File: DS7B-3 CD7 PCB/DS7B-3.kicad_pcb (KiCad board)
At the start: 2 copper layers, 154 x 46.5 mm, 19 parts, among them CON1 Power Connector, CON4 PANASONIC, CON5 SONY, J1 COM. PORT, U2 4040, U3 74LS04, U4 74LS244

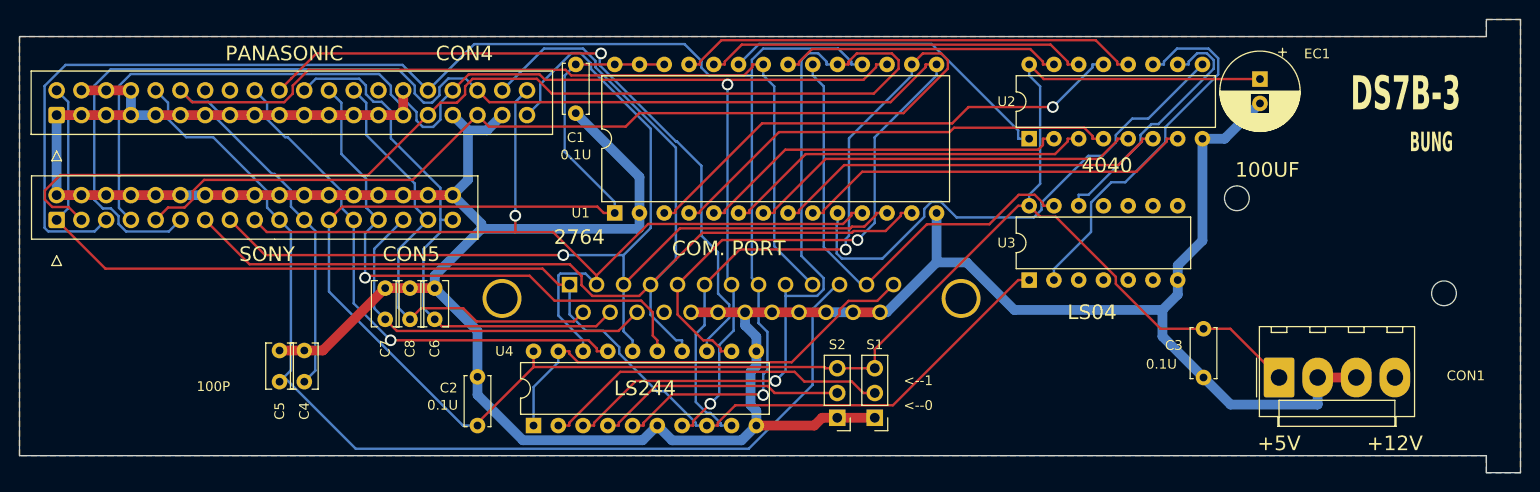
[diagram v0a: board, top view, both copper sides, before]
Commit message: Add files via upload
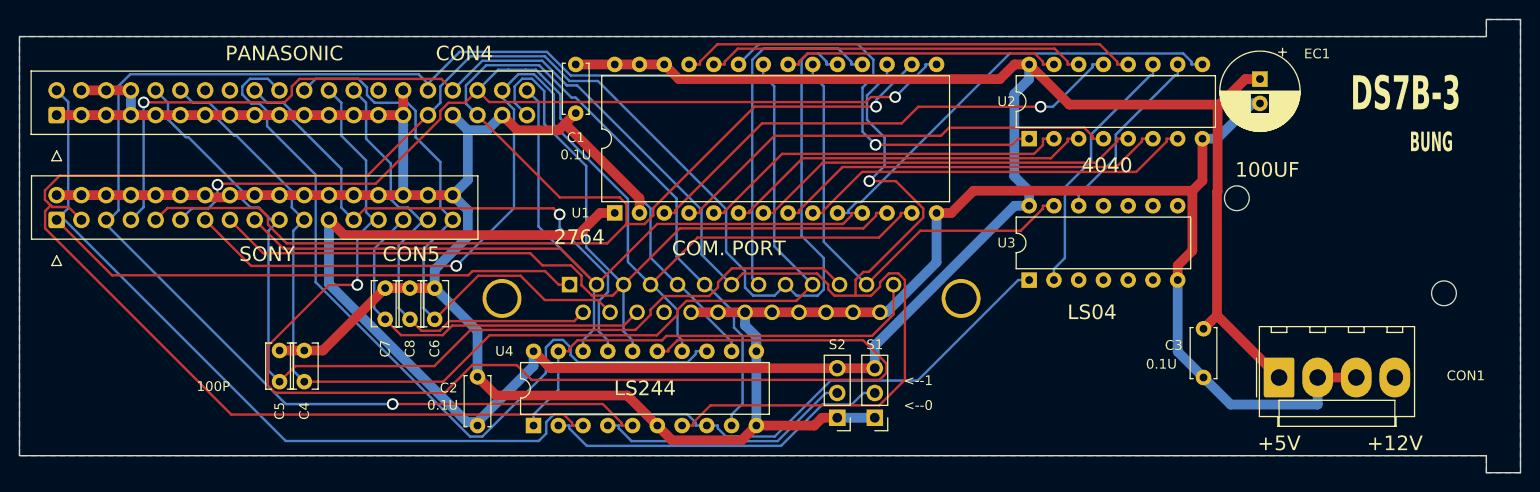
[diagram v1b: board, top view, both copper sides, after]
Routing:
- net /Interrupt: track 57.2 -> 130.8 mm
- net /Reset: track 131.5 -> 188.7 mm
- net /D5: track 139.7 -> 177.6 mm
- net /D3: track 168.2 -> 130.9 mm, vias 1 -> 2
- net /D7: track 173.5 -> 202.5 mm, vias 1 -> 0
- net /+5V: track 227.4 -> 251.0 mm
- net /D6: track 162.5 -> 182.4 mm
- net /D4: track 149.5 -> 168.0 mm
- net /GND: track 353.0 -> 340.4 mm
- net /BinCnt.Reset: track 38.5 -> 26.5 mm
- net /Panasonic.D5: track 71.7 -> 82.7 mm, vias 1 -> 0
- net /D2: track 127.8 -> 117.4 mm, vias 0 -> 1
- net /CD.~{WE}: track 109.3 -> 100.5 mm
- net /A0: track 52.8 -> 45.0 mm
- net /BinCnt.Clk: track 26.3 -> 18.9 mm
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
